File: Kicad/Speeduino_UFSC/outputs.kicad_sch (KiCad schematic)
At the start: 16 parts, among them J2 Conn_01x06, Q2 Q_NMOS_GDSD, Q3 HVM NMOS, U6 ULN2003

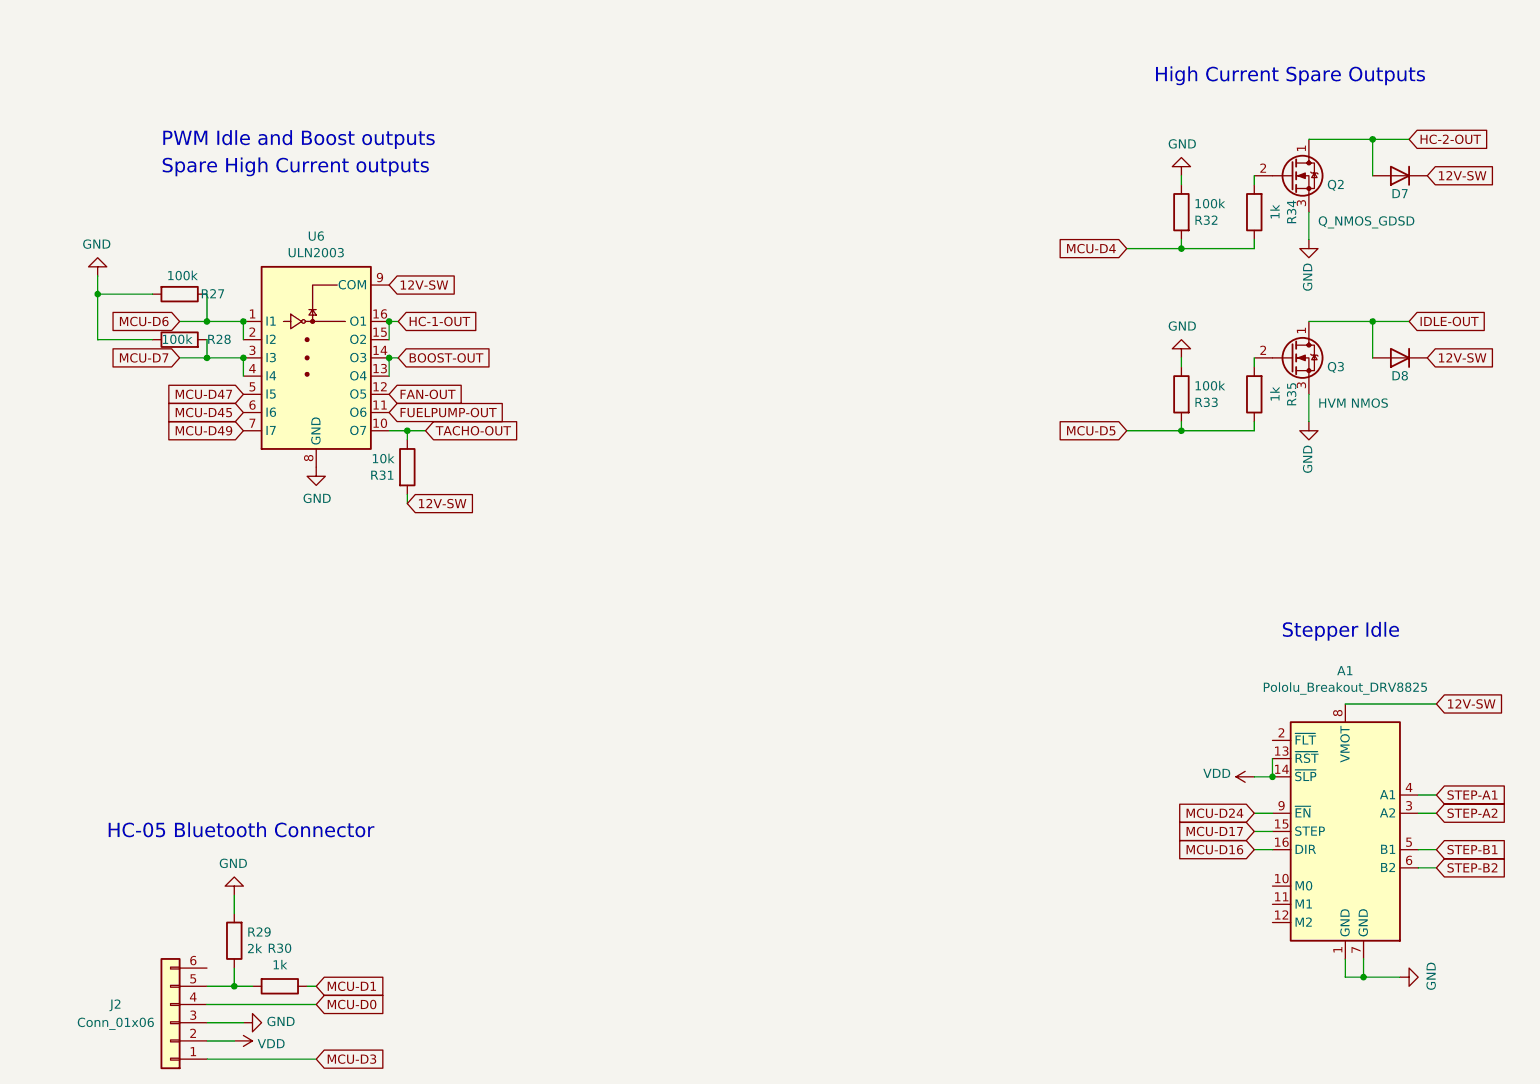
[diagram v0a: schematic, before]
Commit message: Update Kicad
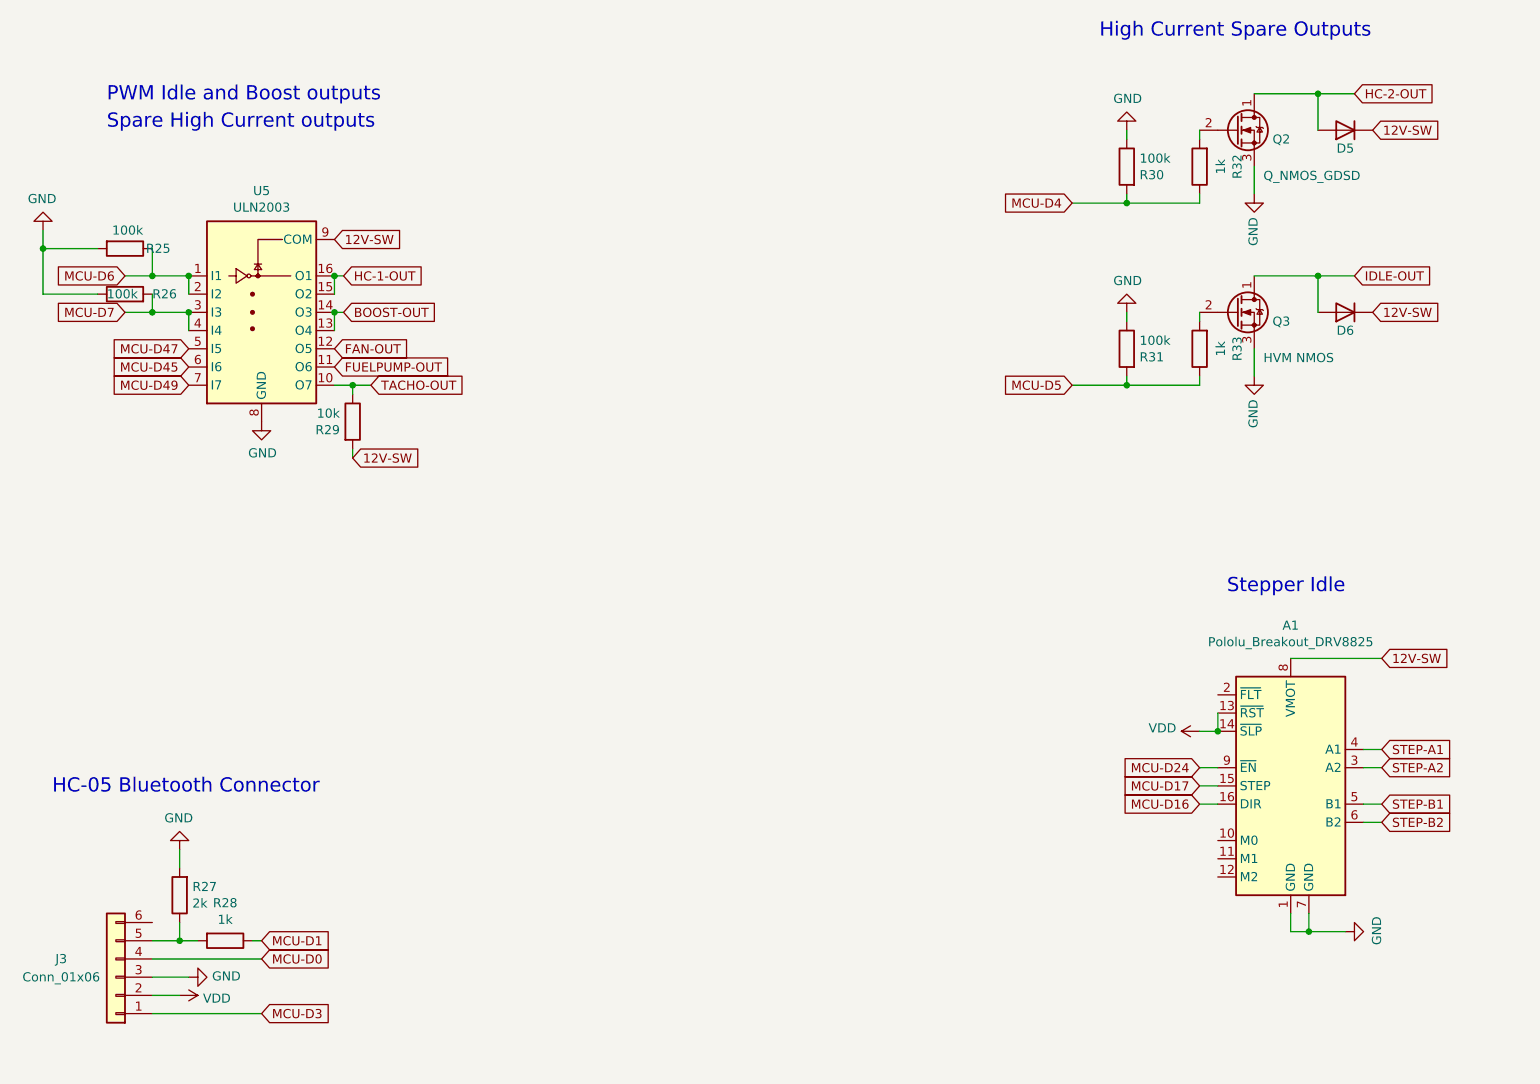
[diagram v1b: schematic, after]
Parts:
- removed D7, D8: D, Diode_THT:D_DO-35_SOD27_P7.62mm_Horizontal, symbol Device:D
- removed J2: Conn_01x06, Connector_PinHeader_2.54mm:PinHeader_1x06_P2.54mm_Vertical, symbol Connector_Generic:Conn_01x06
- removed R34, R35: 1k, Resistor_THT:R_Axial_DIN0204_L3.6mm_D1.6mm_P5.08mm_Horizontal, symbol Device:R
- removed U6: ULN2003, Package_DIP:DIP-16_W7.62mm, symbol Transistor_Array:ULN2003
- added D5, D6: D, Diode_THT:D_DO-35_SOD27_P7.62mm_Horizontal, symbol Device:D
- added J3: Conn_01x06, Connector_PinHeader_2.54mm:PinHeader_1x06_P2.54mm_Vertical, symbol Connector_Generic:Conn_01x06
- added R25, R26: 100k, Resistor_THT:R_Axial_DIN0204_L3.6mm_D1.6mm_P5.08mm_Horizontal, symbol Device:R
- added U5: ULN2003, Package_DIP:DIP-16_W7.62mm, symbol Transistor_Array:ULN2003
- R27: value 100k -> 2k; Digikey Part Number BC3240CT-ND -> BC3254CT-ND; Manufacturer_Part_Number MBA02040C1003FCT00 -> MBA02040C2001FCT00; URL https://www.digikey.com.au/product-detail/en/vishay-beyschlag-draloric-bc-components/MBA02040C1003FCT00/BC3240CT-ND/6138743 -> https://www.digikey.com.au/product-detail/en/vishay-beyschlag-draloric-bc-components/MBA02040C2001FCT00/BC3254CT-ND/6138757
- R28, R32, R33: value 100k -> 1k; Digikey Part Number BC3240CT-ND -> BC1.00KXCT-ND; Manufacturer_Part_Number MBA02040C1003FCT00 -> MBA02040C1001FRP00; URL https://www.digikey.com.au/product-detail/en/vishay-beyschl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 -> (none)
- R29: value 2k -> 10k; Digikey Part Number BC3254CT-ND -> BC10.0KXCT-ND; Manufacturer_Part_Number MBA02040C2001FCT00 -> MBA02040C1002FRP00; URL https://www.digikey.com.au/product-detail/en/vishay-beyschlag-draloric-bc-components/MBA02040C2001FCT00/BC3254CT-ND/6138757 -> https://www.digikey.com.au/product-detail/en/vishay-beyschlag-draloric-bc-components/MBA02040C1002FRP00/BC10-0KXCT-ND/336866
- R30: value 1k -> 100k; Digikey Part Number BC1.00KXCT-ND -> BC3240CT-ND; Manufacturer_Part_Number MBA02040C1001FRP00 -> MBA02040C1003FCT00; URL (none) -> https://www.digikey.com.au/product-detail/en/vishay-beyschl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
- R31: value 10k -> 100k; Digikey Part Number BC10.0KXCT-ND -> BC3240CT-ND; Manufacturer_Part_Number MBA02040C1002FRP00 -> MBA02040C1003FCT00; URL https://www.digikey.com.au/product-detail/en/vishay-beyschlag-draloric-bc-components/MBA02040C1002FRP00/BC10-0KXCT-ND/336866 -> https://www.digikey.com.au/product-detail/en/vishay-beyschlag-draloric-bc-components/MBA02040C1003FCT00/BC3240CT-ND/6138743
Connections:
- net 12V-SW: now also R29.2, D5.1 (K), D6.1 (K), U5.9 (COM); no longer R31.2
- net BOOST-OUT: now also U5.13 (O4), U5.14 (O3)
- net FAN-OUT: now also U5.12 (O5)
- net FUELPUMP-OUT: now also U5.11 (O6)
- net GND: now also R30.1, R31.1, J3.3 (Pin_3), R25.2, R26.1, U5.8 (GND); no longer R28.1, R29.2, R32.1, R33.1
- net HC-1-OUT: now also U5.15 (O2), U5.16 (O1)
- net HC-2-OUT: now also D5.2 (A)
- net IDLE-OUT: now also D6.2 (A)
- net MCU-D0: now also J3.4 (Pin_4)
- net MCU-D1: now also R28.1; no longer R30.1
- net MCU-D3: now also J3.1 (Pin_1)
- net MCU-D4: now also R30.2, R32.1; no longer R32.2
- net MCU-D45: now also U5.6 (I6)
- net MCU-D47: now also U5.5 (I5)
- net MCU-D49: now also U5.7 (I7)
- net MCU-D5: now also R31.2, R33.1; no longer R33.2
- net MCU-D6: now also R25.1, U5.1 (I1), U5.2 (I2); no longer R27.1
- net MCU-D7: now also R26.2, U5.3 (I3), U5.4 (I4); no longer R28.2
- net TACHO-OUT: now also R29.1, U5.10 (O7); no longer R31.1
- net VDD: now also J3.2 (Pin_2)
- net at Q2.2 (G): now also R32.2
- net at Q3.2 (G): now also R33.2
- new net: J3.5 (Pin_5), R27.1, R28.2
